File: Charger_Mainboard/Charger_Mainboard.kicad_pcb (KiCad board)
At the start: 2 copper layers, 104.1 x 114.3 mm, 34 parts, among them J10 Conn_02x10_Odd_Even, J11 Conn_01x02_Pin, J12 Conn_01x02_Pin, J13 Conn_01x02_Pin, J14 Conn_01x02_Pin, J15 Conn_01x02_Pin, J16 Conn_01x02_Pin, J17 Conn_01x02_Pin, J18 DB9_5, J19 DB9_5, J2 Conn_01x02_Pin, J3 Conn_01x02_Pin, J4 Conn_01x02_Pin, J5 Conn_01x02_Pin, J6 Conn_01x02_Pin, J7 Conn_01x02_Pin, J8 DB9_5, U1 AP2204K-ADJ, U2 TLV2371DBV, U3 AP2204K-ADJ

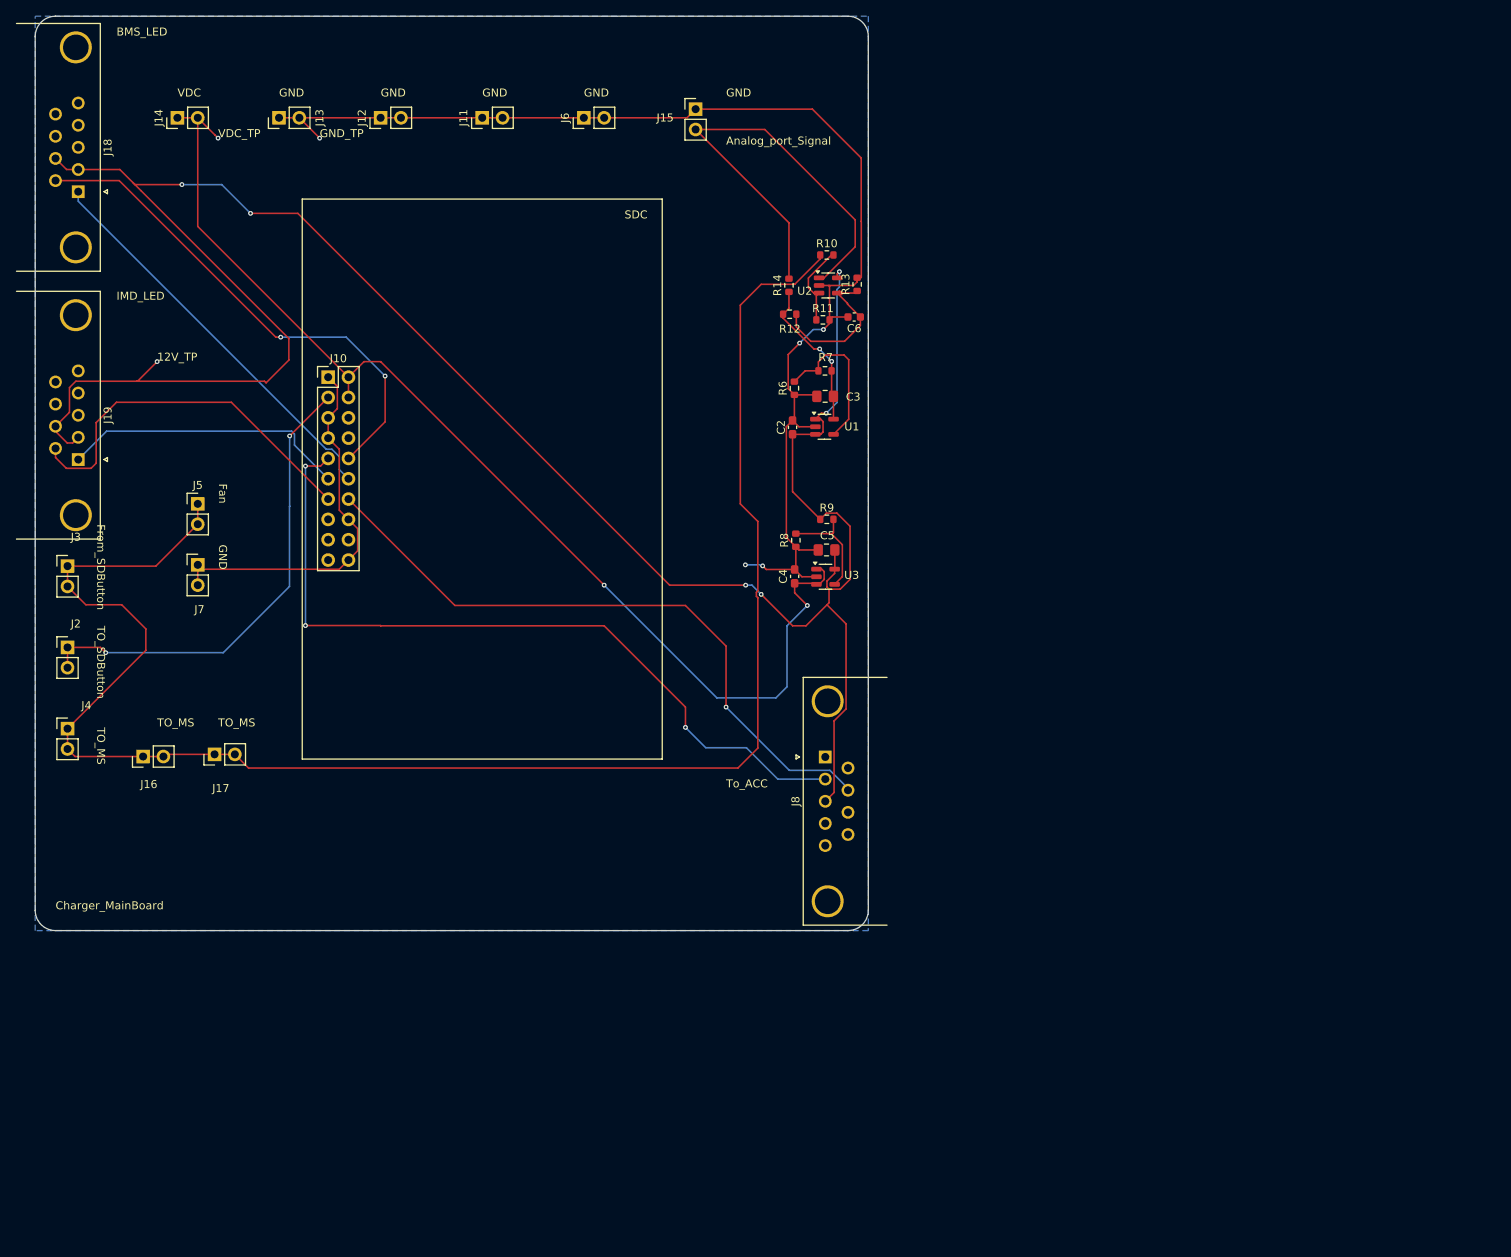
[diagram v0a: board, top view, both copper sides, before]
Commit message: charger mainboard v2025.6
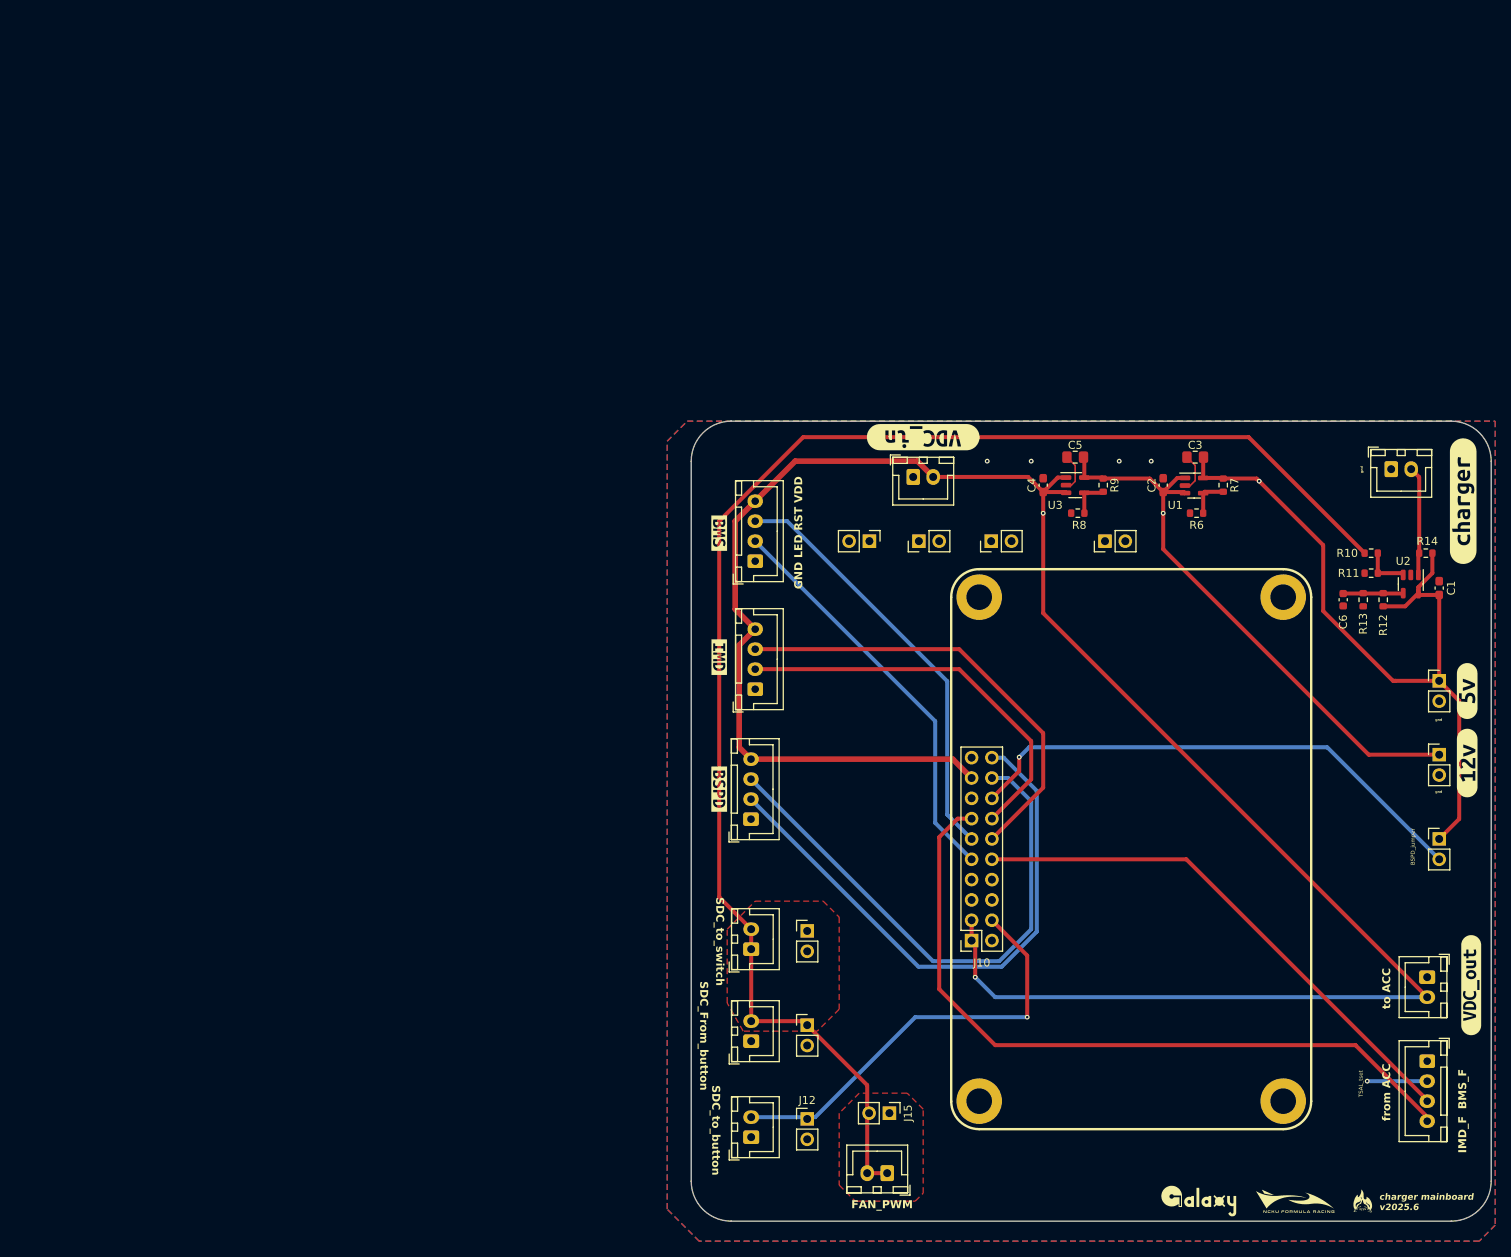
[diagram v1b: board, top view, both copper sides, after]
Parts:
- added C1: 1u, Capacitor_SMD:C_0603_1608Metric_Pad1.08x0.95mm_HandSolder, F.Cu at (175.5, 63.9)
- added G***: LOGO, logo:nckufs_logo_10mm, F.Cu at (157.5, 140.5)
- added G***: LOGO, logo:fire_shark_4mm, F.Cu at (166.0, 140.5)
- added G***: LOGO, logo:galaxy_logo_10mm, F.Cu at (145.5, 140.5)
- added H1: MountingHole_Pad, MountingHole:MountingHole_3.2mm_M3_ISO7380_Pad, F.Cu at (156.0, 65.0)
- added H2: MountingHole_Pad, MountingHole:MountingHole_3.2mm_M3_ISO7380_Pad, F.Cu at (118.0, 128.0)
- added H3: MountingHole_Pad, MountingHole:MountingHole_3.2mm_M3_ISO7380_Pad, F.Cu at (156.0, 128.0)
- added H4: MountingHole_Pad, MountingHole:MountingHole_3.2mm_M3_ISO7380_Pad, F.Cu at (118.0, 65.0)
- added J1: Conn_01x02, Connector_JST:JST_XH_B2B-XH-A_1x02_P2.50mm_Vertical, F.Cu at (109.8, 50.0)
- added J20: Conn_01x02_Pin, Connector_PinHeader_2.54mm:PinHeader_1x02_P2.54mm_Vertical, F.Cu at (104.3, 58.0)
- added J21: Conn_01x04, Connector_JST:JST_XH_B4B-XH-A_1x04_P2.50mm_Vertical, F.Cu at (174.0, 123.0)
- added J22: Conn_01x04, Connector_JST:JST_XH_B4B-XH-A_1x04_P2.50mm_Vertical, F.Cu at (90.0, 60.5)
- added J23: Conn_01x02_Pin, Connector_PinHeader_2.54mm:PinHeader_1x02_P2.54mm_Vertical, F.Cu at (175.5, 95.2)
- added J9: Conn_01x02_Pin, Connector_PinHeader_2.54mm:PinHeader_1x02_P2.54mm_Vertical, F.Cu at (175.5, 84.7)
- added kibuzzard-682D8AF9: G***, kibuzzard-682D8AF9, F.Cu at (85.5, 57.0)
- added kibuzzard-682D8B7A: G***, kibuzzard-682D8B7A, F.Cu at (85.5, 72.5)
- added kibuzzard-68452BF1: G***, kibuzzard-68452BF1, F.Cu at (179.0, 76.7)
- added kibuzzard-68452CD9: G***, kibuzzard-68452CD9, F.Cu at (179.0, 85.7)
- added kibuzzard-68452D38: G***, kibuzzard-68452D38, F.Cu at (111.0, 45.0)
- added kibuzzard-68452D90: G***, kibuzzard-68452D90, F.Cu at (179.5, 113.5)
- added kibuzzard-684531AC: G***, kibuzzard-684531AC, F.Cu at (178.5, 53.0)
- added kibuzzard-68453814: G***, kibuzzard-68453814, F.Cu at (85.5, 89.0)
- J10: footprint Connector_PinHeader_2.54mm:PinHeader_2x10_P2.54mm_Vertical -> Connector_PinSocket_2.54mm:PinSocket_2x10_P2.54mm_Vertical
- J18, J8: value DB9_5 -> Conn_01x04; footprint Connector_Dsub:DSUB-9_Female_Horizontal_P2.77x2.84mm_EdgePinOffset4.94mm_Housed_MountingHolesOffset7.48mm -> Connector_JST:JST_XH_B4B-XH-A_1x04_P2.50mm_Vertical
- J19: value DB9_5 -> Conn_01x02_Pin; footprint Connector_Dsub:DSUB-9_Female_Horizontal_P2.77x2.84mm_EdgePinOffset4.94mm_Housed_MountingHolesOffset7.48mm -> Connector_PinHeader_2.54mm:PinHeader_1x02_P2.54mm_Vertical
- J2, J3, J4, J5, J6, J7: value Conn_01x02_Pin -> Conn_01x02; footprint Connector_PinHeader_2.54mm:PinHeader_1x02_P2.54mm_Vertical -> Connector_JST:JST_XH_B2B-XH-A_1x02_P2.50mm_Vertical
- moved J2 167.0 mm to (169.5, 49.0)
- moved J7 162.1 mm to (174.0, 112.5), turned to -90 degrees
- moved J11 138.8 mm to (175.5, 75.5), turned to 0 degrees
- moved J6 137.3 mm to (106.5, 137.0), turned to 180 degrees
- moved J12 136.0 mm to (96.5, 130.2), turned to 0 degrees
- moved J13 131.2 mm to (96.5, 118.5), turned to 0 degrees
- moved J19 128.8 mm to (133.7, 58.0), turned to 90 degrees
- moved J14 128.6 mm to (96.5, 106.7), turned to 0 degrees
- moved J15 127.8 mm to (106.8, 129.5), turned to -90 degrees
- moved J3 111.3 mm to (89.5, 132.5), turned to 90 degrees
- moved J10 106.9 mm to (117.0, 107.9), turned to 180 degrees
- moved J18 105.0 mm to (90.0, 76.5), turned to 90 degrees
- moved J17 100.7 mm to (119.5, 58.0)
- moved J16 100.6 mm to (110.5, 58.0)
- moved J4 94.0 mm to (89.5, 120.5), turned to 90 degrees
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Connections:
- C4 pad 1: VDC -> BSPD_IN
- J10 pad 1: GND -> BSPD_IN
- J10 pad 10: BMS_LED -> BMS_FAULT
- J10 pad 11: IMD_RST -> BMS_RST
- J10 pad 12: BMS_RST -> IMD_RST
- J10 pad 13: IMD_LED -> IMD_FAULT
- J10 pad 14: IMD_FAULT -> IMD_LED
- J10 pad 15: unconnected-(J10-Pin_15-Pad15) -> GND
- J10 pad 16: GND -> BSPD_FAULT
- J10 pad 17: unconnected-(J10-Pin_17-Pad17) -> BSPD_IN
- J10 pad 18: unconnected-(J10-Pin_18-Pad18) -> BSPD_RST
- J10 pad 19: unconnected-(J10-Pin_19-Pad19) -> GND
- J10 pad 2: VDC -> GND
- J10 pad 20: GND -> BSPD_LED
- J10 pad 3: SDC_TO_SDBUTTON -> BSPD_IN
- J10 pad 4: VDC -> SDC_TO_SDBUTTON
- J10 pad 5: GND -> unconnected-(J10-Pin_5-Pad5)
- J10 pad 6: unconnected-(J10-Pin_6-Pad6) -> GND
- J10 pad 7: GND -> SW_Fault
- J10 pad 8: unconnected-(J10-Pin_8-Pad8) -> GND
- J10 pad 9: BMS_FAULT -> BMS_LED
- J11 pad 1: GND -> +5V
- J12 pad 1: GND -> SDC_TO_SDBUTTON
- J13 pad 1: GND -> FAN_PWM
- J14 pad 1: VDC -> FAN_PWM
- J14 pad 2: VDC -> FAN_PWM
- J15 pad 1: GND -> FAN_PWM
- J15 pad 2: charger_analog -> FAN_PWM
- J16 pad 1: FAN -> GND
- J16 pad 2: FAN -> GND
- J17 pad 1: FAN -> GND
- J17 pad 2: FAN -> GND
- J18 pad 1: BMS_RST -> GND
- J18 pad 2: +12V -> IMD_LED
- J18 pad 3: GND -> IMD_RST
- J18 pad 4: unconnected-(J18-Pad4) -> BSPD_IN
- J19 pad 1: IMD_RST -> GND
- J19 pad 2: +12V -> GND
- J2 pad 1: SDC_TO_SDBUTTON -> GND
- J2 pad 2: SDC_TO_SDBUTTON -> charger_analog
- J3 pad 1: FAN -> GND
- J3 pad 2: FAN -> SDC_TO_SDBUTTON
- J4 pad 1: FAN -> GND
- J4 pad 2: FAN -> FAN_PWM
- J5 pad 1: FAN -> FAN_PWM
- J5 pad 2: FAN -> FAN_PWM
- J6 pad 1: GND -> FAN_PWM
- J6 pad 2: GND -> FAN_PWM
- J7 pad 2: GND -> BSPD_IN
- J8 pad 1: unconnected-(J8-Pad1) -> GND
- J8 pad 2: BMS_FAULT -> BSPD_LED
- J8 pad 3: +12V -> BSPD_RST
- J8 pad 4: unconnected-(J8-Pad4) -> BSPD_IN
- R10 pad 1: FAN -> FAN_PWM
- U2 pad 5: +12V -> +5V
- U3 pad 1: VDC -> BSPD_IN
- U3 pad 3: VDC -> BSPD_IN
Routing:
- net BSPD_IN: track 0.00 -> 258.4 mm, vias 0 -> 2
- net FAN: track 212.4 -> 0.00 mm
- net +12V: track 282.7 -> 71.7 mm, vias 7 -> 1
- net GND: track 208.4 -> 9.68 mm, vias 5 -> 4
- net FAN_PWM: track 0.00 -> 186.8 mm
- net VDC: track 143.2 -> 0.00 mm, vias 4 -> 0
- net +5V: track 19.3 -> 93.4 mm, vias 2 -> 1
- net BSPD_LED: track 0.00 -> 71.8 mm
- net BSPD_RST: track 0.00 -> 68.2 mm
- net BSPD_FAULT: track 0.00 -> 65.4 mm, vias 0 -> 1
- net charger_analog: track 57.6 -> 13.7 mm
- net BMS_FAULT: track 97.6 -> 67.5 mm, vias 3 -> 0
- net IMD_RST: track 36.0 -> 56.2 mm
- net Net-(U1-ADJ): track 19.2 -> 5.07 mm
- net BMS_LED: track 63.5 -> 51.0 mm, vias 2 -> 0
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- added copper zone on F.Cu, net FAN_PWM
- added copper zone on F.Cu, net GND
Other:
- board size 104.1 x 114.3 mm -> 100 x 100 mm
- board text added: "BMS_F"
- board text added: "BSPD_jumper"
- board text added: "FAN_PWM"
- board text added: "GND LED RST VDD"
- board text added: "IMD_F"
- board text added: "SDC_From_button"
- board text added: "SDC_to_button"
- board text added: "SDC_to_switch"
- board text added: "TSAL_tset"
- board text added: "charger mainboard v2025.6"
- board text added: "from ACC"
- board text added: "gnd"
- board text added: "to ACC"
- board text removed: "12V_TP"
- board text removed: "Analog_port_Signal"
- board text removed: "BMS_LED"
- board text removed: "Charger_MainBoard"
- board text removed: "Fan"
- board text removed: "From_SDButton"
- board text removed: "GND"
- board text removed: "GND_TP"
- board text removed: "IMD_LED"
- board text removed: "SDC"
- board text removed: "TO_MS"
- board text removed: "TO_SDButton"
- board text removed: "To_ACC"
- board text removed: "VDC"
- board text removed: "VDC_TP"
